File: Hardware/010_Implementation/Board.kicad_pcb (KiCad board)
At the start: 2 copper layers, 170 x 75 mm, 66 parts, among them IC1 SN65HVD233-HT, J1 2606-3356, J2 JTAG Jumper Pins, J3 DSUB9, K1 G5V-2-DC5, K2 G5V-2-DC5, Q1 BC817, SW1 SW_Push, U1 TPS62160DGK, U2 ESP32-DEVKITC-32D

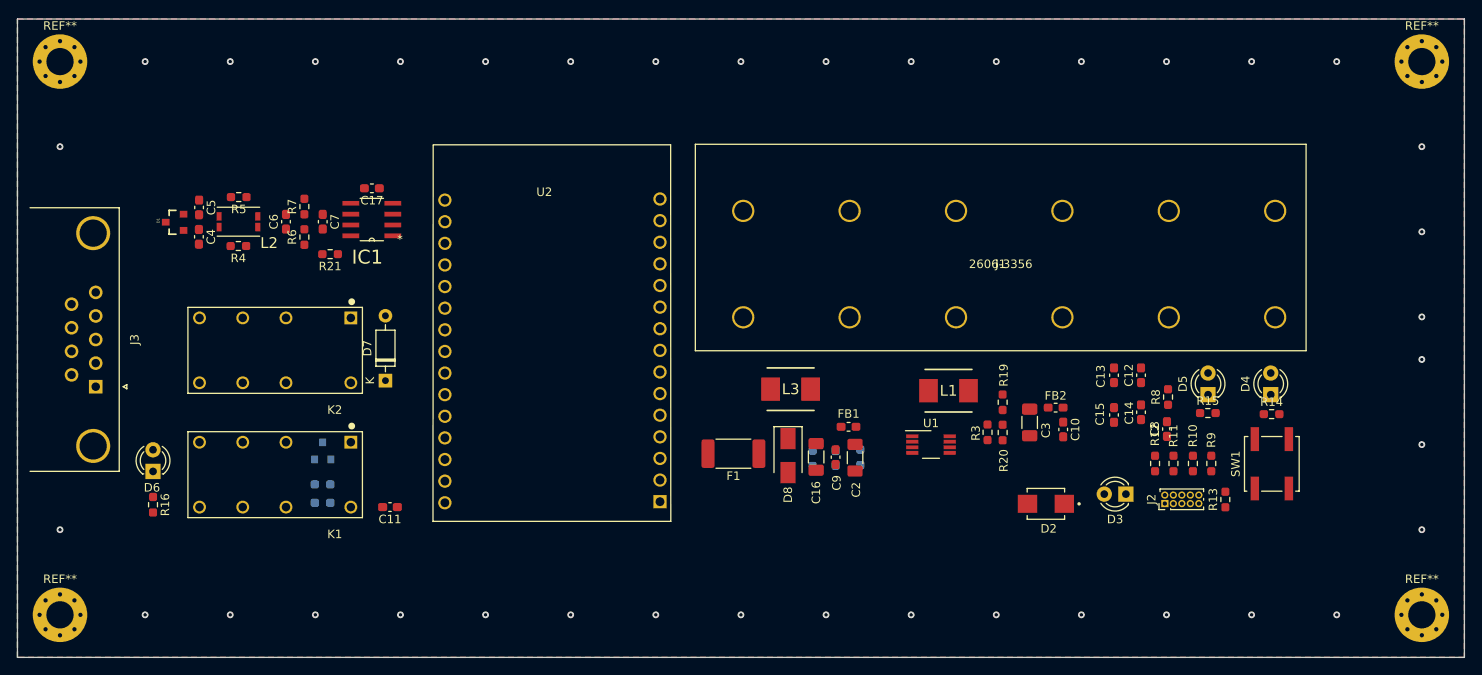
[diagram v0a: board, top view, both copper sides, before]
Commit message: Board Version 7
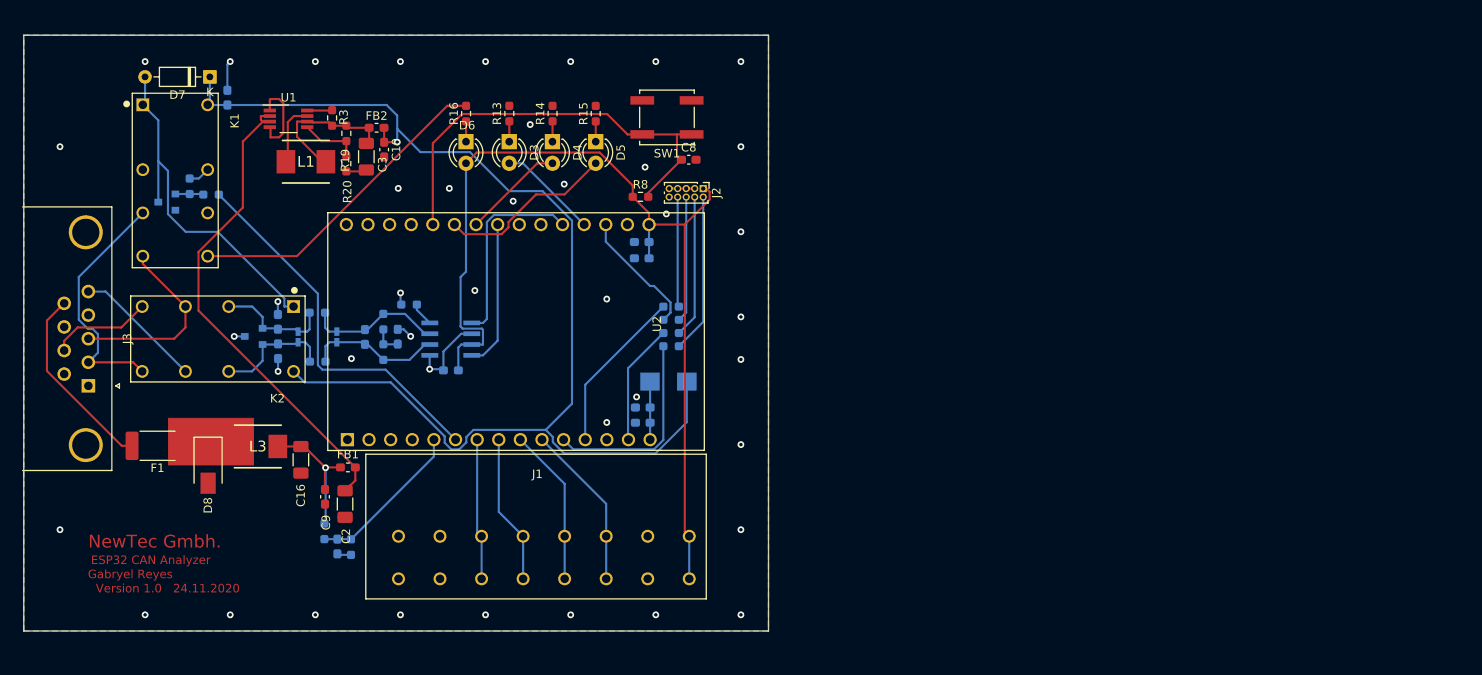
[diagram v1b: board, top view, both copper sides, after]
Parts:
- removed REF** (x4): MountingHole_3.2mm_M3_Pad_Via, MountingHole:MountingHole_3.2mm_M3_Pad_Via
- C11, C12, C13, C14, C15, C17, C4, C5, C6, C7, D1, D2, IC1, L2, R10, R11, R12, R21, R4, R5, R6, R7, R9: moved to B.Cu
- J1: value 2606-3356 -> Conn_01x08_Female; footprint Board:2606-3356 -> Board:AST 045-08
- moved R13 95.6 mm to (96.1, 67.6)
- moved R14 91.6 mm to (101.2, 67.6), turned to 90 degrees
- moved D4 89.5 mm to (101.2, 70.9), turned to 270 degrees
- moved C10 86.3 mm to (81.4, 71.8)
- moved FB2 86.3 mm to (80.5, 69.2)
- moved R3 85.4 mm to (75.3, 68.1), turned to 90 degrees
- moved U1 84.6 mm to (70.2, 68.2)
- moved C3 84.0 mm to (79.3, 72.6)
- moved D3 83.4 mm to (96.1, 70.9), turned to 270 degrees
- moved R19 83.3 mm to (76.9, 69.9), turned to 270 degrees
- moved R20 83.3 mm to (76.9, 73.4)
- moved SW1 81.9 mm to (114.6, 68.0), turned to 0 degrees
- moved L1 80.1 mm to (72.2, 73.2)
- moved R15 80.1 mm to (106.2, 67.6), turned to 90 degrees
- moved D5 77.8 mm to (106.2, 70.9), turned to 270 degrees
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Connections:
- J1 pad 1: (no net) -> +3V3
- J1 pad 2: /MCU/GPIO_1 -> GND
- J1 pad 3: (no net) -> /MCU/GPIO_1
- J1 pad 5: (no net) -> /MCU/GPIO_3
- J1 pad 6: /MCU/GPIO_3 -> /MCU/GPIO_4
- J1 pad 8: /MCU/GPIO_4 -> (no net)
- K2 pad 11: /Connector/Pin_3 -> /Connector/Pin_5
- K2 pad 13: /CAN_Transceiver/BUS_H -> /CAN_Transceiver/BUS_L
- K2 pad 4: /CAN_Transceiver/BUS_L -> /CAN_Transceiver/BUS_H
- K2 pad 6: /Connector/Pin_5 -> /Connector/Pin_3
- K2 pad 8: /Connector/Pin_2 -> /Connector/Pin_7
- K2 pad 9: /Connector/Pin_7 -> /Connector/Pin_2
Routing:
- net +5V: track 0.00 -> 143.0 mm, vias 0 -> 1
- net +3V3: track 0.00 -> 112.8 mm
- net Net-(C2-Pad1): track 0.00 -> 58.1 mm
- net /MCU/WiFi_Mode: track 0.00 -> 51.5 mm
- net /Connector/~OBD~\CAN: track 0.00 -> 44.7 mm
- net Net-(D7-Pad2): track 0.00 -> 42.1 mm
- net GND: track 0.00 -> 40.7 mm, vias 38 -> 42
- net /Connector/CAN_Mode: track 0.00 -> 37.7 mm
- net /Connector/Pin_2: track 0.00 -> 29.2 mm
- net /MCU/MTMS: track 0.00 -> 23.7 mm
- net /CAN_Transceiver/CAN_Tx: track 0.00 -> 23.1 mm
- net /Connector/OBD_VDD: track 0.00 -> 22.4 mm
- net /Connector/Pin_3: track 0.00 -> 22.4 mm
- net /MCU/Indicator_STA_Mode: track 0.00 -> 20.9 mm
- net /MCU/GPIO_1: track 0.00 -> 19.5 mm
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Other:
- board size 170 x 75 mm -> 87.5 x 70 mm
- board text added: "ESP32 CAN Analyzer"
- board text added: "Gabryel Reyes"
- board text added: "NewTec Gmbh."
- board text added: "Version 1.0 24.11.2020"
- board text removed: "I/O"
- board text removed: "~OBD~\CAN Switch"
